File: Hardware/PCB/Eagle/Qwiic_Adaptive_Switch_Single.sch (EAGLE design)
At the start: 11 parts, among them J2 J2, SW1 CUI_SJ1-3513, SW2 CUI_SJ1-3513

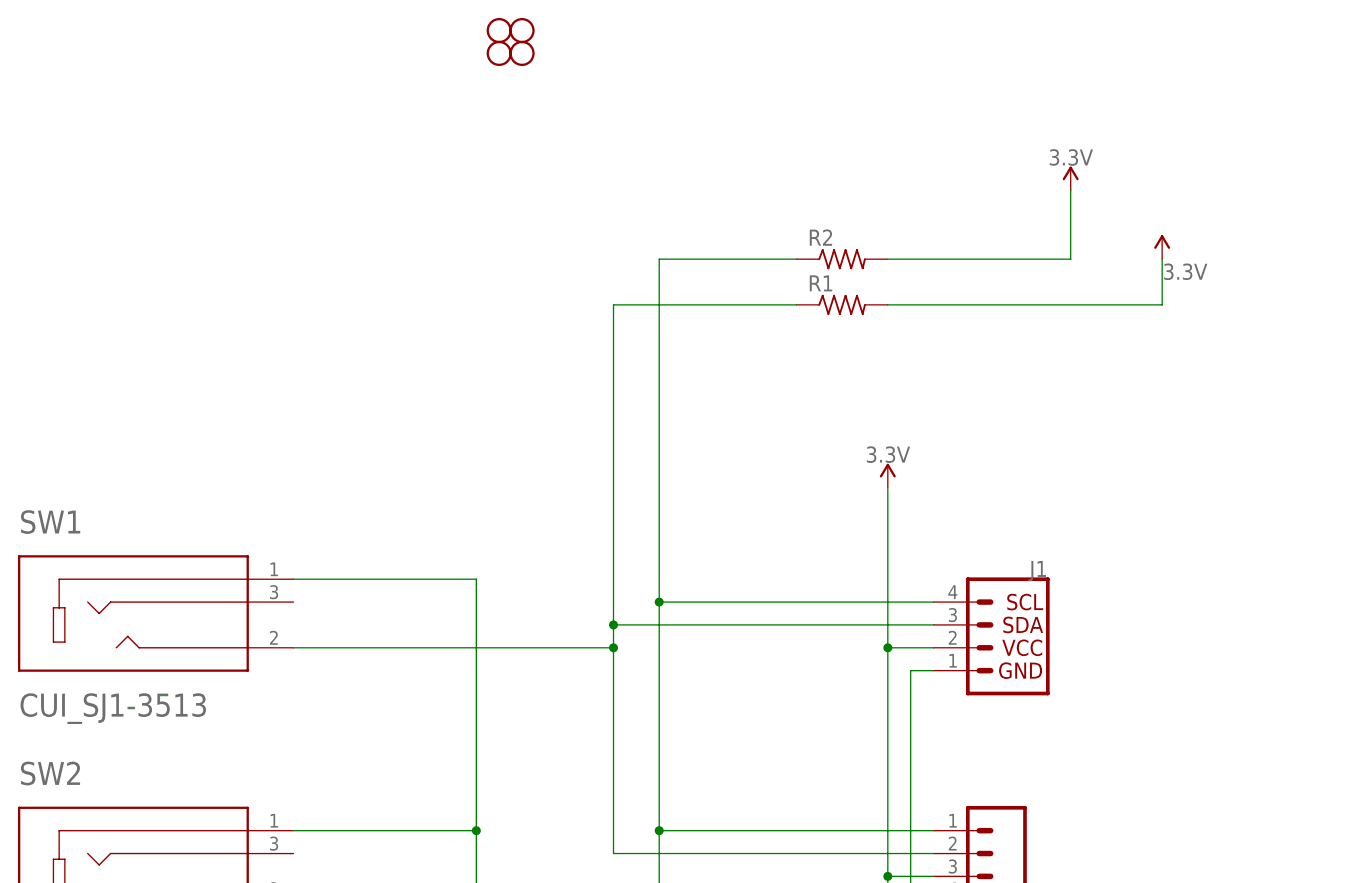
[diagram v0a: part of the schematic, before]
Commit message: Updated the design.
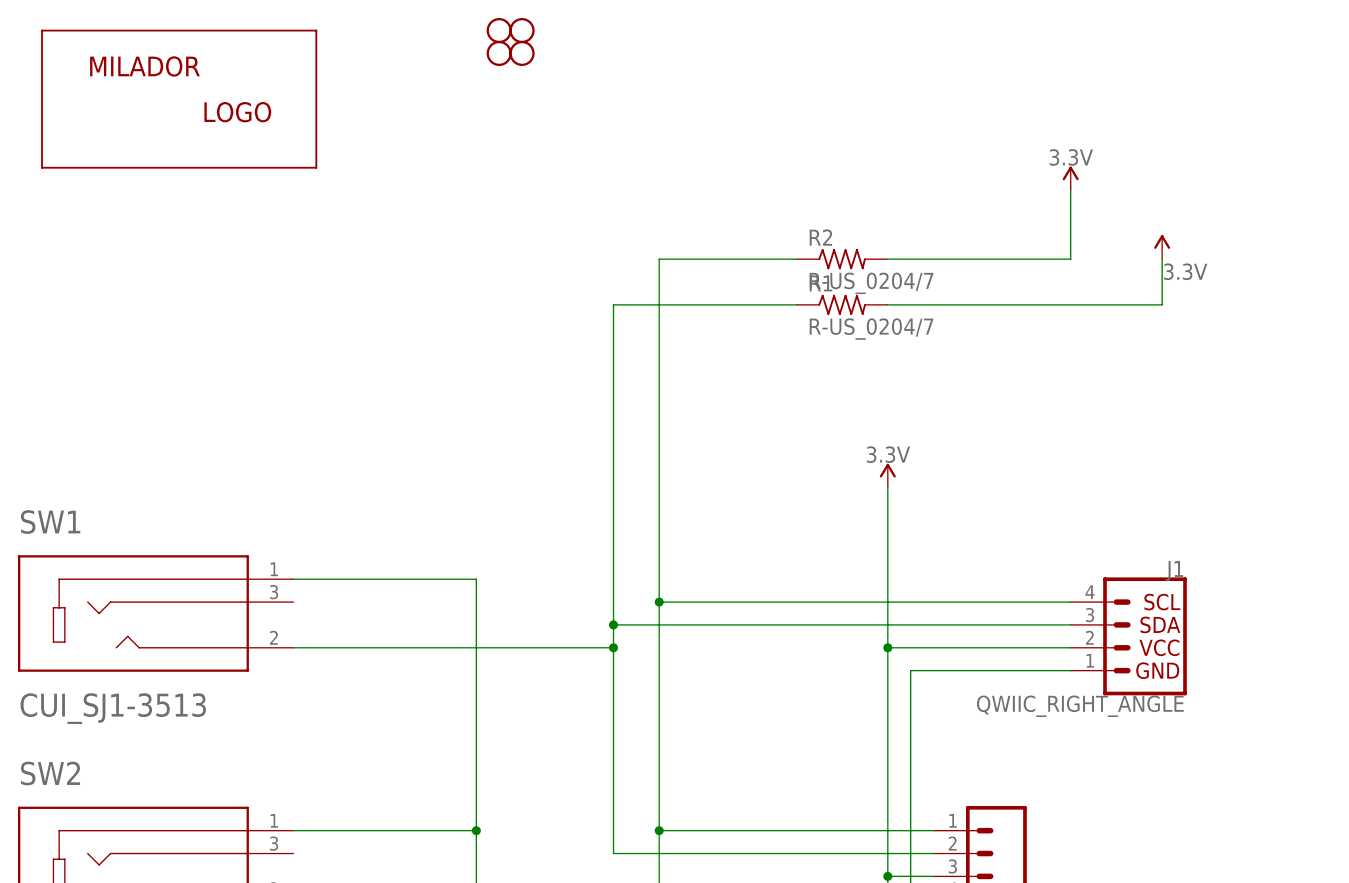
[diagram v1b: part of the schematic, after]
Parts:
- added U$2: MILADOR-LOGO-, milador:MILADOR-LOGO-
- J1: value (none) -> QWIIC_RIGHT_ANGLE; device SparkFun-Connectors:QWIIC_CONNECTORJS-1MM -> milador_SMD:QWIIC_CONNECTORSJS-1MM
- J2, J3: device SparkFun-Connectors:CONN_041X04_NO_SILK_NO_POP -> milador:CONNECTORS_CONN_041X04_NO_SILK
- R1, R2: value (none) -> R-US_0204/7; device MMC Eagle:RESISTOR-US-0204/7 -> milador:R-US_0204/7
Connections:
- net 3.3V: now also J1.2; no longer J1.VCC
- net GND: now also J1.1; no longer J1.GND
- net SCL/SCK: now also J1.4; no longer J1.SCL
- net SDA/MOSI: now also J1.3; no longer J1.SDA
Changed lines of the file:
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@@
 <layer number="154" name="FabDoc2" color="7" fill="1" visible="yes" active="yes"/>
 <layer number="155" name="FabDoc3" color="7" fill="1" visible="yes" active="yes"/>
+<layer number="160" name="O_Dim" color="7" fill="1" visible="no" active="yes"/>
 <layer number="166" name="AntennaArea" color="7" fill="1" visible="yes" active="yes"/>
 <layer number="168" name="4mmHeightArea" color="7" fill="1" visible="yes" active="yes"/>
@@
 <parts>
 <part name="SUPPLY6" library="SparkFun-PowerSymbols" deviceset="3.3V" device="" value="3.3V"/>
-<part name="J1" library="SparkFun-Connectors" library_urn="urn:adsk.eagle:library:513" deviceset="QWIIC_CONNECTOR" device="JS-1MM" package3d_urn="urn:adsk.eagle:package:38096/1"/>
 <part name="JP3" library="SparkFun-Hardware" deviceset="STAND-OFF" device=""/>
 <part name="JP4" library="SparkFun-Hardware" deviceset="STAND-OFF" device=""/>
 <part name="JP2" library="SparkFun-Hardware" deviceset="STAND-OFF" device=""/>
 <part name="GND8" library="SparkFun-PowerSymbols" deviceset="GND" device=""/>
-<part name="J2" library="SparkFun-Connectors" deviceset="CONN_04" device="1X04_NO_SILK_NO_POP" value="J2"/>
+<part name="J2" library="milador" library_urn="urn:adsk.eagle:library:12595918" deviceset="CONNECTORS_CONN_04" device="1X04_NO_SILK" package3d_urn="urn:adsk.eagle:package:29222251/2" value="J2"/>
 <part name="GND18" library="SparkFun-PowerSymbols" deviceset="GND" device=""/>
 <part name="SW2" library="MMC Eagle" library_urn="urn:adsk.eagle:library:13126479" deviceset="CUI_SJ1-3513" device="" package3d_urn="urn:adsk.eagle:package:25599488/3"/>
 <part name="SW1" library="MMC Eagle" library_urn="urn:adsk.eagle:library:13126479" deviceset="CUI_SJ1-3513" device="" package3d_urn="urn:adsk.eagle:package:25599488/3"/>
-<part name="J3" library="SparkFun-Connectors" deviceset="CONN_04" device="1X04_NO_SILK_NO_POP"/>
+<part name="J3" library="milador" library_urn="urn:adsk.eagle:library:12595918" deviceset="CONNECTORS_CONN_04" device="1X04_NO_SILK" package3d_urn="urn:adsk.eagle:package:29222251/2"/>
 <part name="SUPPLY1" library="SparkFun-PowerSymbols" deviceset="3.3V" device="" value="3.3V"/>
 <part name="SUPPLY2" library="SparkFun-PowerSymbols" deviceset="3.3V" device="" value="3.3V"/>
-<part name="R1" library="MMC Eagle" library_urn="urn:adsk.eagle:library:13126479" deviceset="RESISTOR-US-" device="0204/7" package3d_urn="urn:adsk.eagle:package:13126612/3"/>
-<part name="R2" library="MMC Eagle" library_urn="urn:adsk.eagle:library:13126479" deviceset="RESISTOR-US-" device="0204/7" package3d_urn="urn:adsk.eagle:package:13126612/3"/>
+<part name="R1" library="milador" library_urn="urn:adsk.eagle:library:12595918" deviceset="R-US_0204/7" device="" package3d_urn="urn:adsk.eagle:package:23498/2"/>
+<part name="R2" library="milador" library_urn="urn:adsk.eagle:library:12595918" deviceset="R-US_0204/7" device="" package3d_urn="urn:adsk.eagle:package:23498/2"/>
 <part name="FRAME1" library="frames" library_urn="urn:adsk.eagle:library:229" deviceset="A4L-LOC" device=""/>
 <part name="JP1" library="SparkFun-Hardware" library_urn="urn:adsk.eagle:library:519" deviceset="STAND-OFF" device="" package3d_urn="urn:adsk.eagle:package:38630/1"/>
+<part name="J1" library="milador_SMD" library_urn="urn:adsk.eagle:library:27847482" deviceset="QWIIC_CONNECTORS" device="JS-1MM" package3d_urn="urn:adsk.eagle:package:29222212/3" value="QWIIC_RIGHT_ANGLE"/>
+<part name="U$2" library="milador" library_urn="urn:adsk.eagle:library:12595918" deviceset="MILADOR-LOGO-" device="" package3d_urn="urn:adsk.eagle:package:28431737/1"/>
 </parts>
 <sheets>
@@
 <attribute name="VALUE" x="472.44" y="89.154" size="1.778" layer="96" align="bottom-center"/>
 </instance>
-<instance part="J1" gate="J1" x="485.14" y="68.58" smashed="yes" rot="MR0">
-<attribute name="NAME" x="490.22" y="76.454" size="1.778" layer="95" font="vector" rot="MR0"/>
-</instance>
 <instance part="JP3" gate="G$1" x="429.26" y="137.16" smashed="yes"/>
 <instance part="JP4" gate="G$1" x="429.26" y="134.62" smashed="yes"/>
@@
 </instance>
 <instance part="JP1" gate="G$1" x="431.8" y="137.16" smashed="yes"/>
+<instance part="J1" gate="G$1" x="500.38" y="68.58" smashed="yes" rot="MR0">
+<attribute name="VALUE" x="505.46" y="63.246" size="1.778" layer="96" font="vector" rot="MR0" align="top-left"/>
+<attribute name="NAME" x="505.46" y="76.454" size="1.778" layer="95" font="vector" rot="MR0"/>
+</instance>
+<instance part="U$2" gate="G$1" x="393.7" y="129.54" smashed="yes"/>
 </instances>
 <busses>
@@
 <net name="GND" class="0">
 <segment>
-<pinref part="J1" gate="J1" pin="GND"/>
-<wire x1="477.52" y1="66.04" x2="474.98" y2="66.04" width="0.1524" layer="91"/>
 <wire x1="477.52" y1="40.64" x2="474.98" y2="40.64" width="0.1524" layer="91"/>
 <pinref part="GND8" gate="1" pin="GND"/>
@@
 <wire x1="477.52" y1="20.32" x2="474.98" y2="20.32" width="0.1524" layer="91"/>
 <junction x="474.98" y="20.32"/>
+<pinref part="J1" gate="G$1" pin="1"/>
+<wire x1="492.76" y1="66.04" x2="474.98" y2="66.04" width="0.1524" layer="91"/>
 </segment>
 <segment>
@@
 <pinref part="J2" gate="J1" pin="2"/>
 <wire x1="477.52" y1="45.72" x2="441.96" y2="45.72" width="0.1524" layer="91"/>
-<pinref part="J1" gate="J1" pin="SDA"/>
-<wire x1="477.52" y1="71.12" x2="441.96" y2="71.12" width="0.1524" layer="91"/>
+<wire x1="492.76" y1="71.12" x2="441.96" y2="71.12" width="0.1524" layer="91"/>
 <pinref part="R1" gate="G$1" pin="1"/>
 <wire x1="462.28" y1="106.68" x2="441.96" y2="106.68" width="0.1524" layer="91"/>
@@
 <wire x1="441.96" y1="45.72" x2="441.96" y2="68.58" width="0.1524" layer="91"/>
 <junction x="441.96" y="68.58"/>
+<pinref part="J1" gate="G$1" pin="3"/>
 </segment>
 </net>
@@
 <segment>
 <pinref part="J2" gate="J1" pin="1"/>
-<pinref part="J1" gate="J1" pin="SCL"/>
-<wire x1="477.52" y1="73.66" x2="447.04" y2="73.66" width="0.1524" layer="91"/>
+<wire x1="492.76" y1="73.66" x2="447.04" y2="73.66" width="0.1524" layer="91"/>
 <wire x1="447.04" y1="73.66" x2="447.04" y2="111.76" width="0.1524" layer="91"/>
 <pinref part="R2" gate="G$1" pin="1"/>
@@
 <wire x1="477.52" y1="48.26" x2="447.04" y2="48.26" width="0.1524" layer="91"/>
 <junction x="447.04" y="48.26"/>
+<pinref part="J1" gate="G$1" pin="4"/>
 </segment>
 </net>
@@
 <wire x1="477.52" y1="43.18" x2="472.44" y2="43.18" width="0.1524" layer="91"/>
 <pinref part="SUPPLY6" gate="G$1" pin="3.3V"/>
-<pinref part="J1" gate="J1" pin="VCC"/>
-<wire x1="477.52" y1="68.58" x2="472.44" y2="68.58" width="0.1524" layer="91"/>
 <wire x1="472.44" y1="68.58" x2="472.44" y2="86.36" width="0.1524" layer="91"/>
 <wire x1="472.44" y1="43.18" x2="472.44" y2="68.58" width="0.1524" layer="91"/>
@@
 <wire x1="472.44" y1="22.86" x2="472.44" y2="43.18" width="0.1524" layer="91"/>
 <junction x="472.44" y="43.18"/>
-</segment>
-<segment>
+<pinref part="J1" gate="G$1" pin="2"/>
+<wire x1="492.76" y1="68.58" x2="472.44" y2="68.58" width="0.1524" layer="91"/>
+</segment>
+<segment>
